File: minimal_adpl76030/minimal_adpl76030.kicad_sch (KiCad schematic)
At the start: 6 parts, among them Q1 60 V, Q2 60 V, Q3 25 V, Q4 25 V, U1 ADPL76030EUFD-PBF

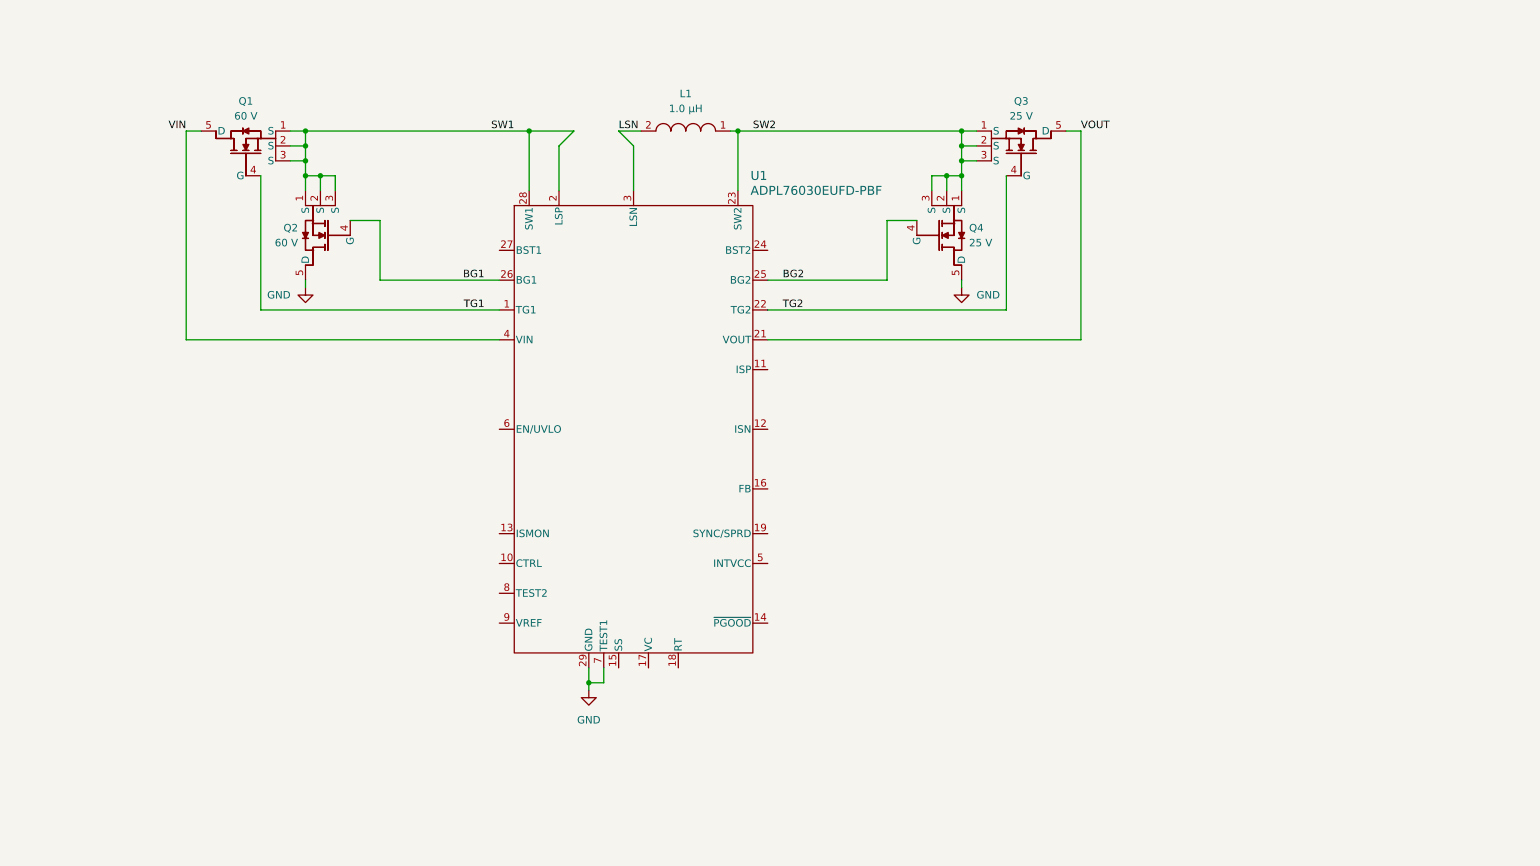
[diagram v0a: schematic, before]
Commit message: backup
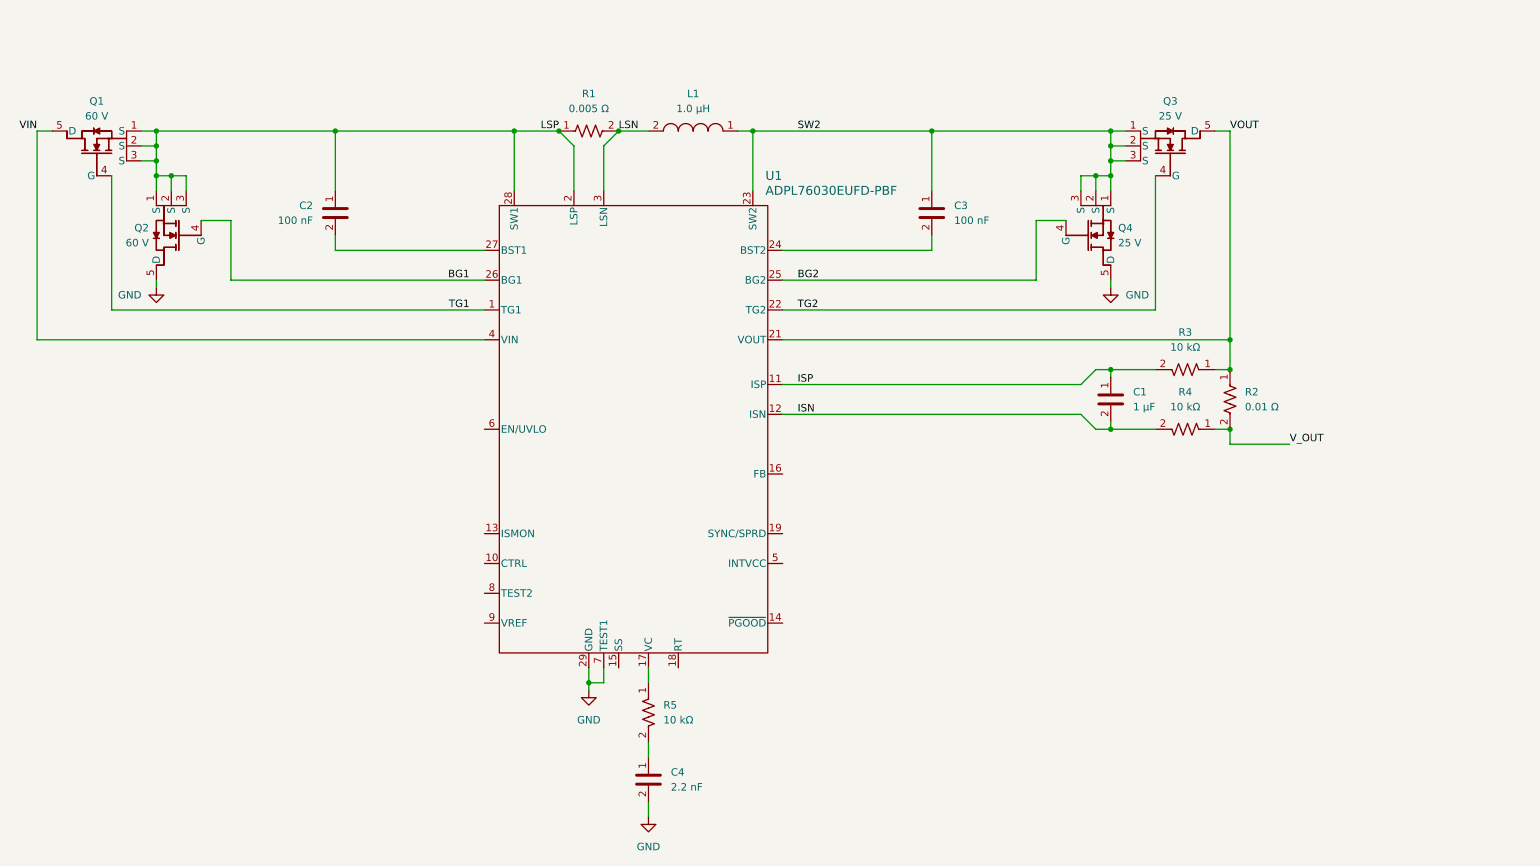
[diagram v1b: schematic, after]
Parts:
- added C1: 1 µF, capacitor_footprints:C_0402_1005Metric, symbol CAPACITORS_C1005X6S1C_DATA_BASE:C_C1005X6S1C105K050BC
- added C2, C3: 100 nF, capacitor_footprints:C_0402_1005Metric, symbol CAPACITORS_GCM155R71H_DATA_BASE:C_GCM155R71H104KE02D
- added C4: 2.2 nF, capacitor_footprints:C_0402_1005Metric, symbol CAPACITORS_GCM155R71H_DATA_BASE:C_GCM155R71H222KA37D
- added R1: 0.005 Ω, resistor_footprints:R_2010_5025Metric, symbol RESISTORS_CRF2010-FZ-_DATA_BASE:R_CRF2010-FZ-R005ELF
- added R2: 0.01 Ω, resistor_footprints:R_2010_5025Metric, symbol RESISTORS_CRF2010-FZ-_DATA_BASE:R_CRF2010-FZ-R010ELF
- added R3, R4, R5: 10 kΩ, resistor_footprints:R_0402_1005Metric, symbol RESISTORS_ERJ-2RKF_DATA_BASE:R_ERJ-2RKF1002X
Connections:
- net GND: now also C4.2
- net LSN: now also R1.2
- net SW2: now also C3.1
- net VOUT: now also R2.1, R3.1
- net ISP: now reaches U1.11 (ISP)
- net ISP: now also C1.1, R3.2
- net ISN: now reaches U1.12 (ISN)
- net ISN: now also C1.2, R4.2
- net at U1.17 (VC): now also R5.1
- net at U1.24 (BST2): now also C3.2
- net at U1.27 (BST1): now also C2.2
- net SW1 renamed LSP
- net LSP: now also C2.1, R1.1
- new net: C4.1, R5.2
- new net V_OUT: R2.2, R4.1
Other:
- moved on the sheet: L1, Q1, Q2, Q3, Q4

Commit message: backup
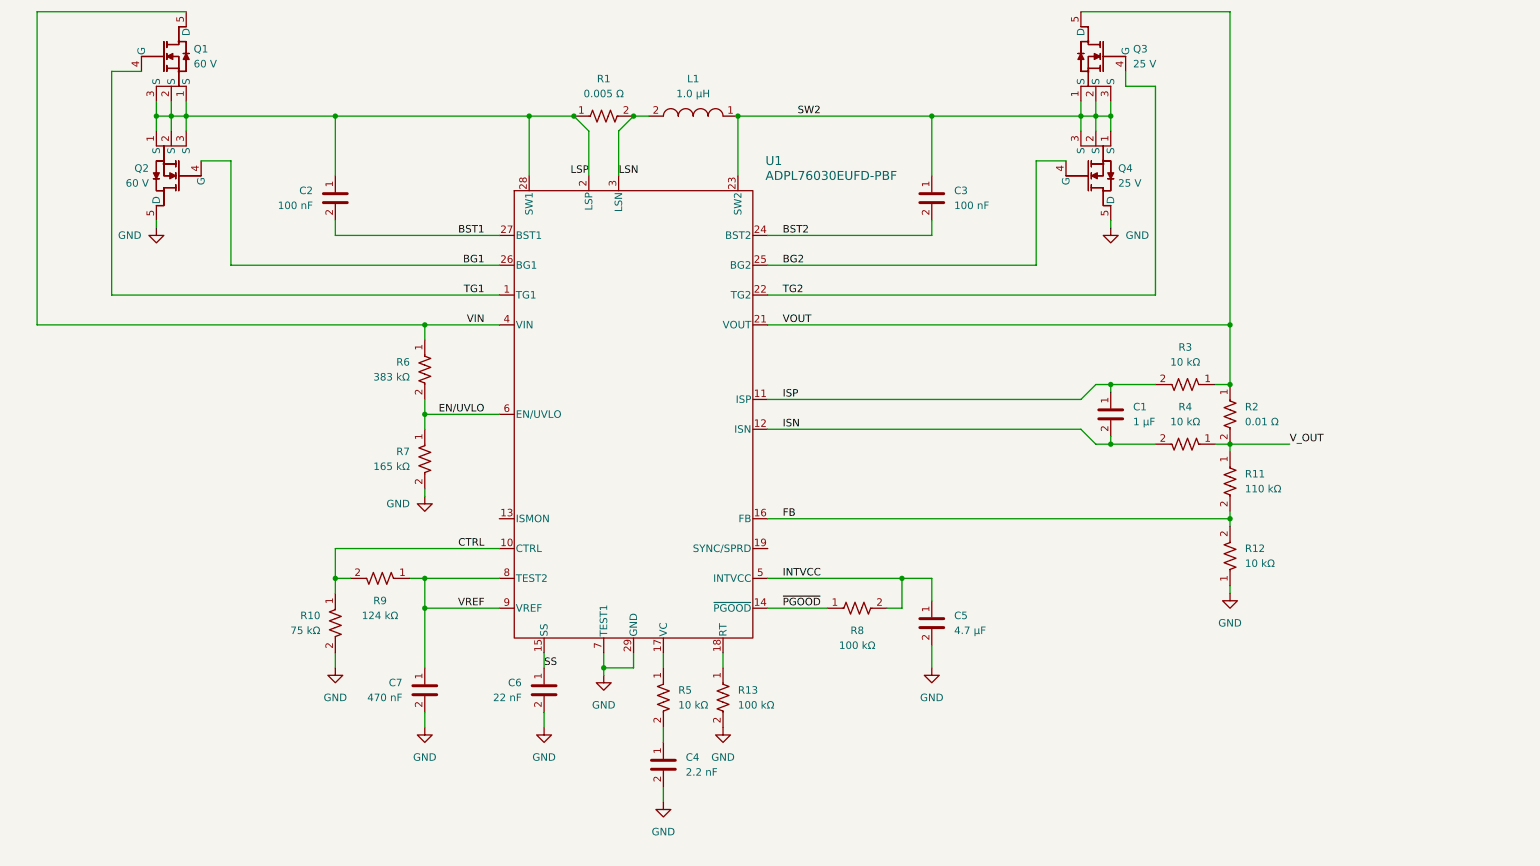
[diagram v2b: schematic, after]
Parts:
- added C5: 4.7 µF, capacitor_footprints:C_0603_1608Metric, symbol CAPACITORS_GRM188C71A_DATA_BASE:C_GRM188C71A475KE11D
- added C6: 22 nF, capacitor_footprints:C_0402_1005Metric, symbol CAPACITORS_GCM155R71H_DATA_BASE:C_GCM155R71H223KA55D
- added C7: 470 nF, capacitor_footprints:C_0402_1005Metric, symbol CAPACITORS_GCM155C71A_DATA_BASE:C_GCM155C71A474KE36D
- added R10: 75 kΩ, resistor_footprints:R_0402_1005Metric, symbol RESISTORS_ERJ-2RKF_DATA_BASE:R_ERJ-2RKF7502X
- added R11: 110 kΩ, resistor_footprints:R_0402_1005Metric, symbol RESISTORS_ERJ-2RKF_DATA_BASE:R_ERJ-2RKF1103X
- added R12: 10 kΩ, resistor_footprints:R_0402_1005Metric, symbol RESISTORS_ERJ-2RKF_DATA_BASE:R_ERJ-2RKF1002X
- added R13, R8: 100 kΩ, resistor_footprints:R_0402_1005Metric, symbol RESISTORS_ERJ-2RKF_DATA_BASE:R_ERJ-2RKF1003X
- added R6: 383 kΩ, resistor_footprints:R_0402_1005Metric, symbol RESISTORS_ERJ-2RKF_DATA_BASE:R_ERJ-2RKF3833X
- added R7: 165 kΩ, resistor_footprints:R_0402_1005Metric, symbol RESISTORS_ERJ-2RKF_DATA_BASE:R_ERJ-2RKF1653X
- added R9: 124 kΩ, resistor_footprints:R_0402_1005Metric, symbol RESISTORS_ERJ-2RKF_DATA_BASE:R_ERJ-2RKF1243X
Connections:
- net GND: now also C5.2, C6.2, C7.2, R10.2, R12.1, R13.2, R7.2
- net VIN: now also R6.1
- net V_OUT: now also R11.1
- net BST1: now reaches C2.2, U1.27 (BST1)
- net BST2: now reaches C3.2, U1.24 (BST2)
- net CTRL: now reaches U1.10 (CTRL)
- net CTRL: now also R10.1, R9.2
- net ~{PGOOD}: now reaches U1.14 (~{PGOOD})
- net ~{PGOOD}: now also R8.1
- net SS: now reaches U1.15 (SS)
- net SS: now also C6.1
- net FB: now reaches U1.16 (FB)
- net FB: now also R11.2, R12.2
- net at U1.18 (RT): now also R13.1
- net INTVCC: now reaches U1.5 (INTVCC)
- net INTVCC: now also C5.1, R8.2
- net EN/UVLO: now reaches U1.6 (EN/UVLO)
- net EN/UVLO: now also R6.2, R7.1
- net VREF: now reaches U1.8 (TEST2)
- net VREF: now also U1.9 (VREF), C7.1, R9.1
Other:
- moved on the sheet: C1, C2, C3, C4, L1, Q1, Q2, Q3, Q4, R1, R2, R3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

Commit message: backup
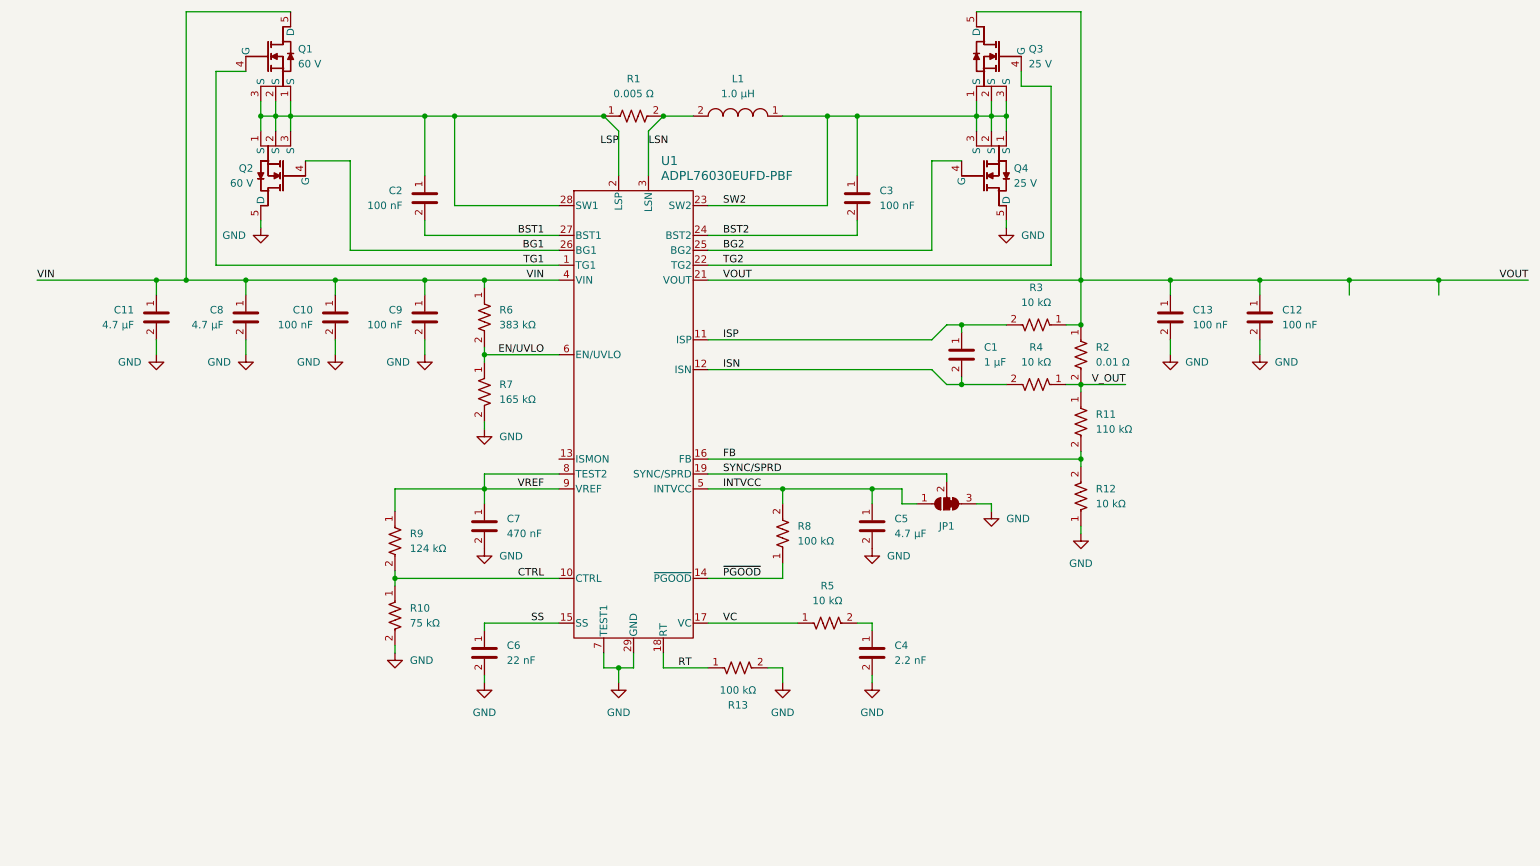
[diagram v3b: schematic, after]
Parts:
- added C10, C12, C13, C9: 100 nF, capacitor_footprints:C_0402_1005Metric, symbol CAPACITORS_GCM155R71H_DATA_BASE:C_GCM155R71H104KE02D
- added C11, C8: 4.7 µF, capacitor_footprints:C_1206_3216Metric, symbol CAPACITORS_CL31B_DATA_BASE:C_CL31B475KBHNNN#
- added JP1: SolderJumper_3_Open, solder_jumper_footprints:SolderJumper-3_P1.3mm_Bridged_2_3_RoundedPad1.0x1.5mm_NumberLabels_1, symbol UNITED_SOLDER_JUMPERS:SolderJumper_3_Bridged_2_3
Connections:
- net GND: now also C10.2, C11.2, C12.2, C13.2, C8.2, C9.2, JP1.3 (B)
- net INTVCC: now also JP1.1 (A)
- net VIN: now also C10.1, C11.1, C8.1, C9.1
- net VOUT: now also C12.1, C13.1
- net RT: now reaches R13.1, U1.18 (RT)
- net VC: now reaches R5.1, U1.17 (VC)
- net SYNC/SPRD: now reaches U1.19 (SYNC/SPRD)
- net SYNC/SPRD: now also JP1.2 (C)
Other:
- moved on the sheet: C1, C2, C3, C4, C5, C6, C7, L1, Q1, Q2, Q3, Q4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
